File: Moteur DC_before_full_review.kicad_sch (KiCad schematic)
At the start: 10 parts, among them J5 Conn_01x04_Pin, U2 DRV8874PWPR

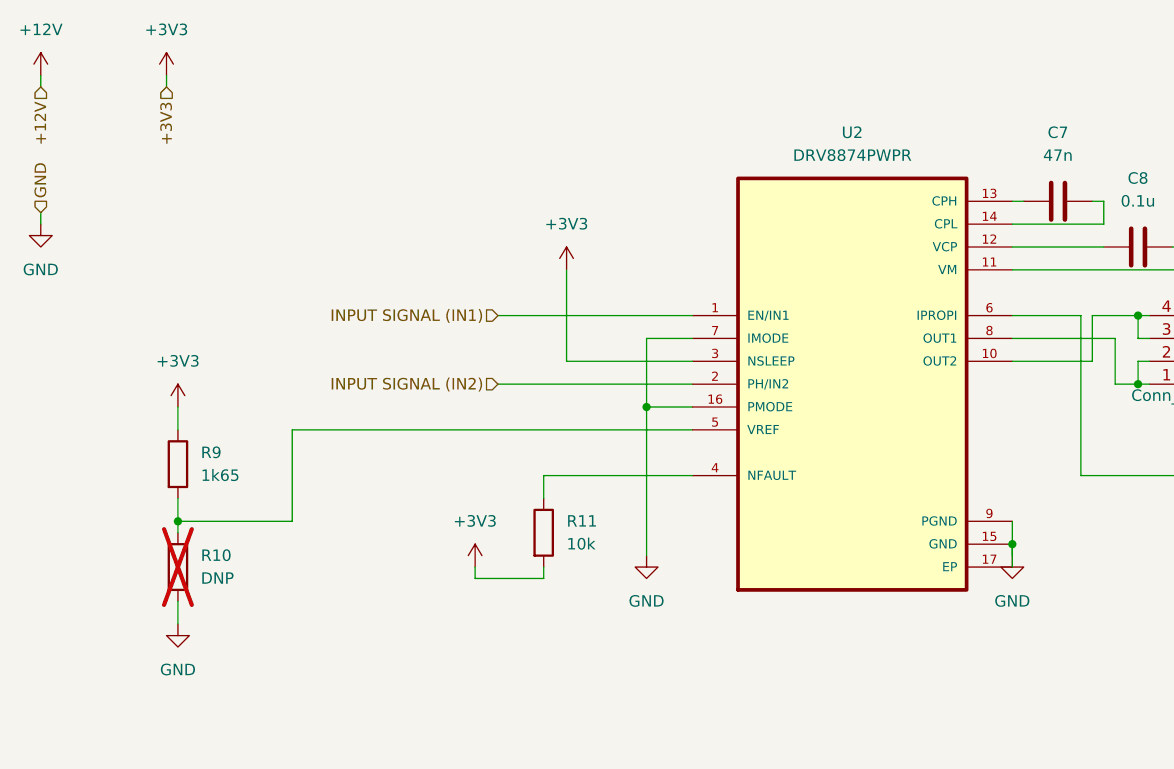
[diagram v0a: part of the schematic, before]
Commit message: Yes
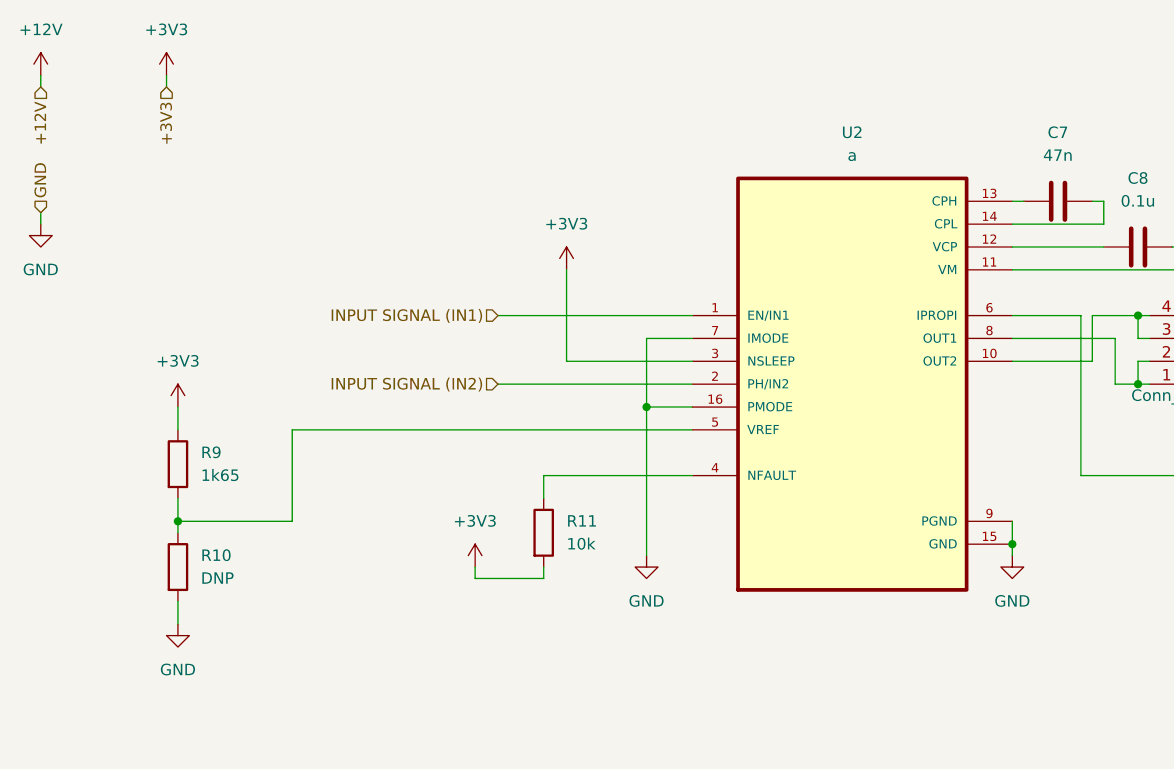
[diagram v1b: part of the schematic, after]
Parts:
- R10: now fitted
- U2: value DRV8874PWPR -> a; symbol Rework_local:DRV8874PWPR_EP17 -> DRV8874:DRV8874PWPR
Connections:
- net GND: no longer U2.17 (EP)
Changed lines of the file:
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@@
 		(on_board yes)
 		(in_pos_files yes)
-		(dnp yes)
+		(dnp no)
 		(fields_autoplaced yes)
 		(property "Reference" "R10"
@@
 	)
 	(symbol
-		(lib_id "Rework_local:DRV8874PWPR_EP17")
+		(lib_id "DRV8874:DRV8874PWPR")
 		(at 128.27 76.2 0)
 		(unit 1)
@@
 			)
 		)
-		(property "Value" "DRV8874PWPR"
+		(property "Value" "a"
 			(at 128.27 50.8 0)
 			(show_name no)
@@
 			)
 		)
-		(property "Datasheet" "https://www.ti.com/lit/ds/symlink/drv8874.pdf"
+		(property "Datasheet" ""
 			(at 128.27 76.2 0)
 			(hide yes)
@@
 			)
 		)
-(pin "17")
-)
+	)
 	(symbol
 		(lib_id "power:+5V")
@@
 		)
 	)
-(wire (pts (xy 146.0500 93.9800) (xy 146.0500 96.5200)) (stroke (width 0) (type default)))
 )
